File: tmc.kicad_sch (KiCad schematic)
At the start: 29 parts, among them J7 Screw_Terminal_01x04, U6 TMC5160A-TA

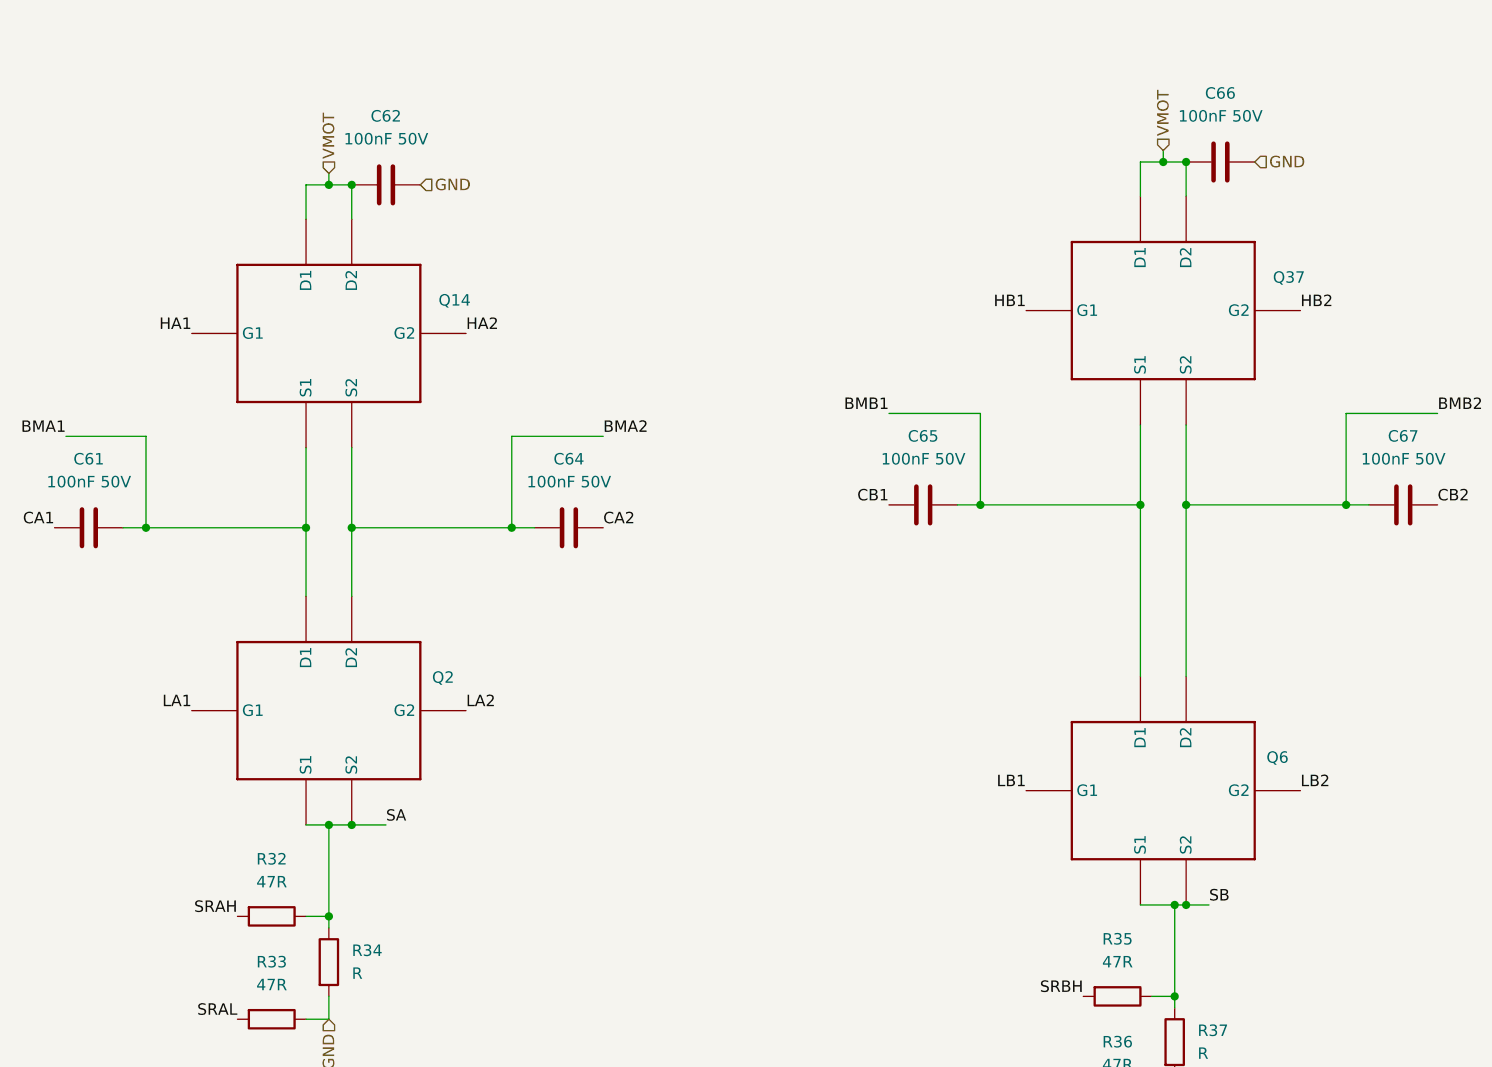
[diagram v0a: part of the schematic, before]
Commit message: first stepper unit
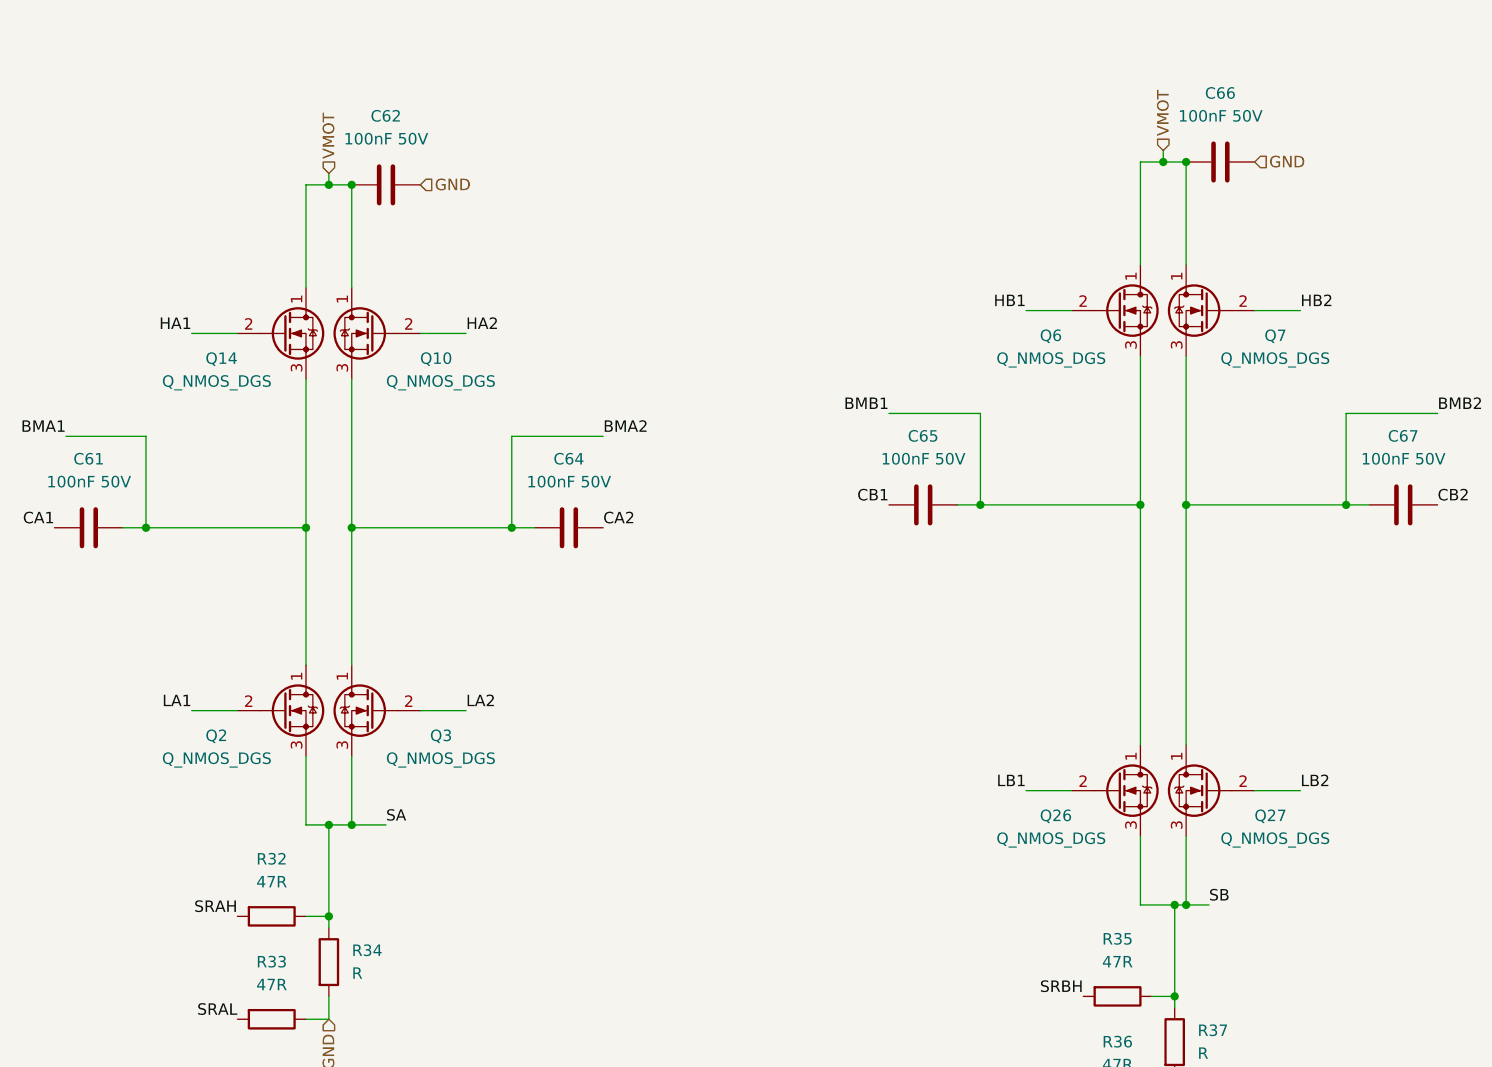
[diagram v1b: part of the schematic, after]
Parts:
- removed Q14, Q2, Q37, Q6: ~, easyeda2kicad:POWERPAK-SO-8_L6.2-W5.2-P1.27-BL_POWERPAK, symbol FET:SQJB70EP-T1_GE3
- added Q10, Q14, Q2, Q26, Q27, Q3, Q6, Q7: Q_NMOS_DGS, FET:Diodes_DMT6016LFDF, symbol Device:Q_NMOS_DGS
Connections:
- net BMA1: now also Q14.3 (S), Q2.1 (D)
- net BMA2: now also Q10.3 (S), Q3.1 (D)
- net BMB1: now also Q26.1 (D), Q6.3 (S)
- net BMB2: now also Q27.1 (D), Q7.3 (S)
- net HA1: now also Q14.2 (G)
- net HA2: now also Q10.2 (G)
- net HB1: now also Q6.2 (G)
- net HB2: now also Q7.2 (G)
- net LA1: now also Q2.2 (G)
- net LA2: now also Q3.2 (G)
- net LB1: now also Q26.2 (G)
- net LB2: now also Q27.2 (G)
- net SA: now also Q2.3 (S), Q3.3 (S)
- net SB: now also Q26.3 (S), Q27.3 (S)
- net VMOT: now also Q10.1 (D), Q14.1 (D), Q6.1 (D), Q7.1 (D)
